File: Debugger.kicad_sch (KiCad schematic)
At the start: 20 parts, among them J101 USB_B_Mini, J102 Conn_01x06_Pin, SW101 SW_SPDT, U101 STM32F103C8Tx

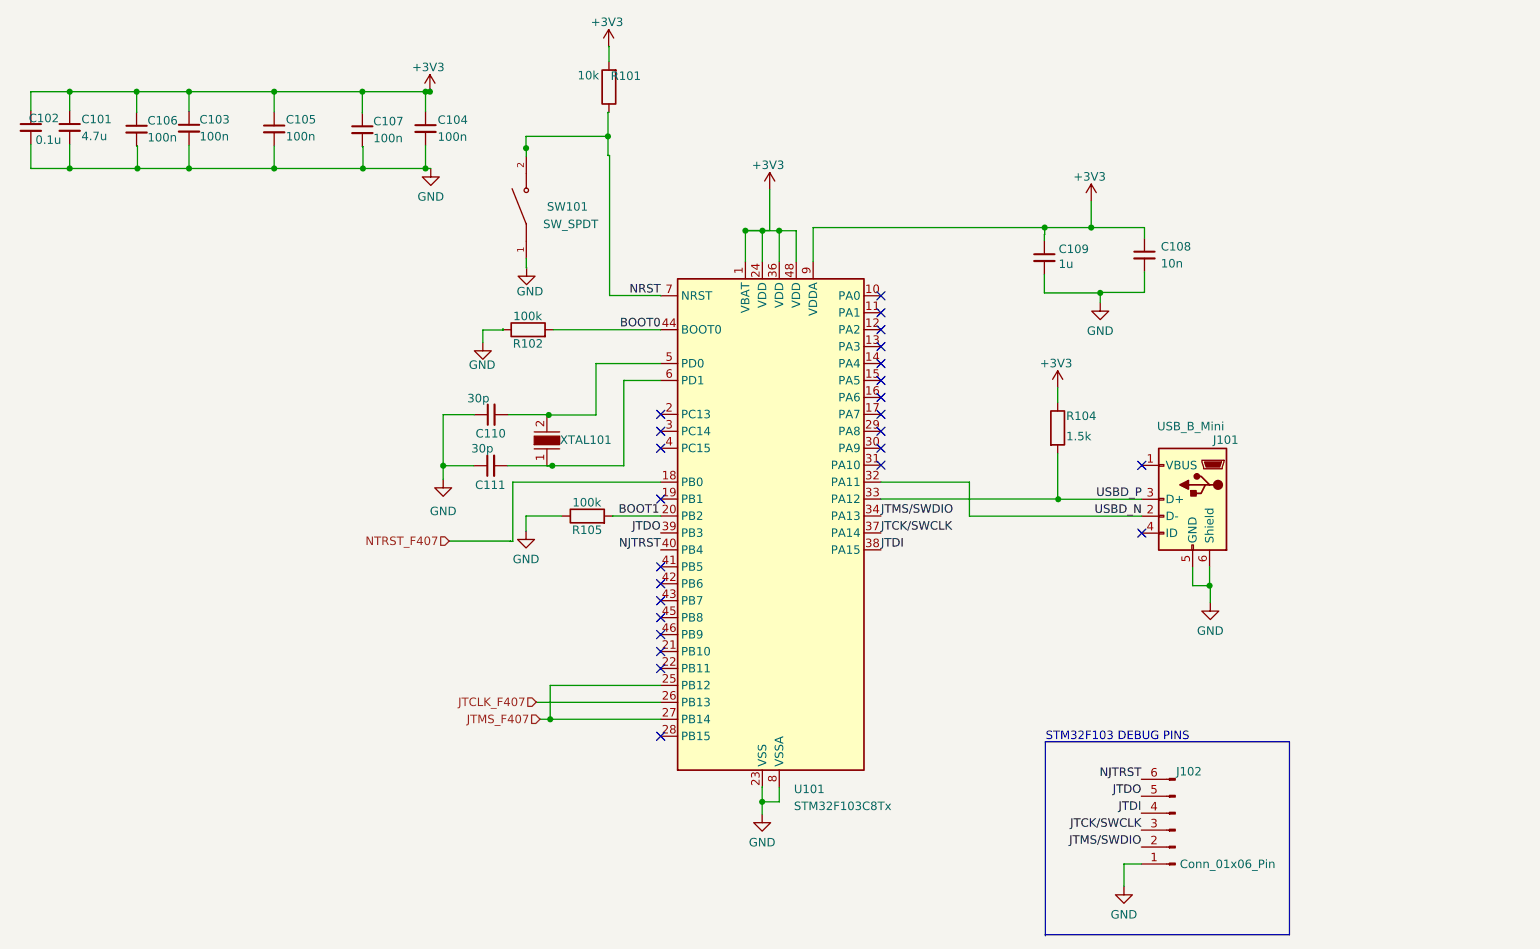
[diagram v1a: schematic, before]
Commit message: schematic pages are reviewed
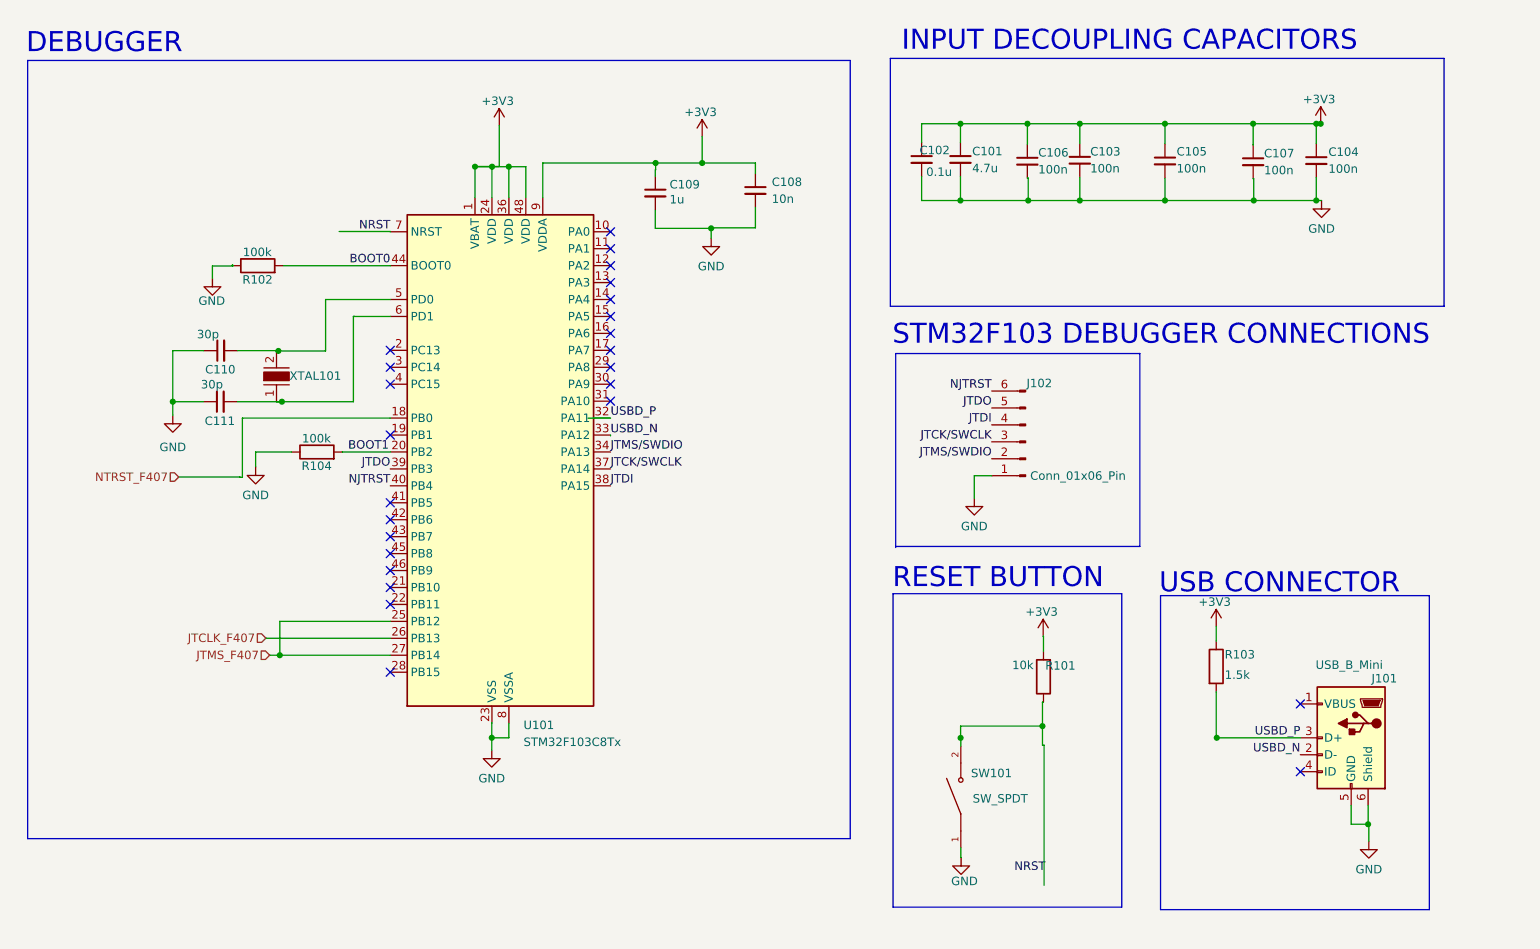
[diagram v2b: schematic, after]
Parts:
- renumbered R104 to R103, R105 to R104
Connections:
- net NRST: no longer R101.1, SW101.2
- net USBD_N: now also U101.33 (PA12); no longer U101.32 (PA11)
- net USBD_P: now also U101.32 (PA11); no longer U101.33 (PA12)
- new net: R101.1, SW101.2
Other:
- note added: "DEBUGGER"
- note added: "INPUT DECOUPLING CAPACITORS"
- note added: "RESET BUTTON"
- note added: "STM32F103 DEBUGGER CONNECTIONS"
- note added: "USB CONNECTOR"
- note removed: "STM32F103 DEBUG PINS"
- moved on the sheet: C101, C102, C103, C104, C105, C106, C107, C108, C109, C110, C111, J101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
